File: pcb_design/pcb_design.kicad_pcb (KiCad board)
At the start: 2 copper layers, 37 parts, among them J1 USB_C_Receptacle_USB2.0_16P, J2 JST_PH_S2B-PH-K, J3 JST_PH_S2B-PH-K, J4 JST_PH_S2B-PH-K, Q1 MMBT3904, Q2 MMBT3904, SW1 SW_SPDT, U1 AP2112K-3.3, U2 ESP32-C3-WROOM-02, U3 MPU-6050, U4 QMC6308, U5 AP2112K-1.8, U6 TXS0102DCU, U7 MCP73831-2-OT

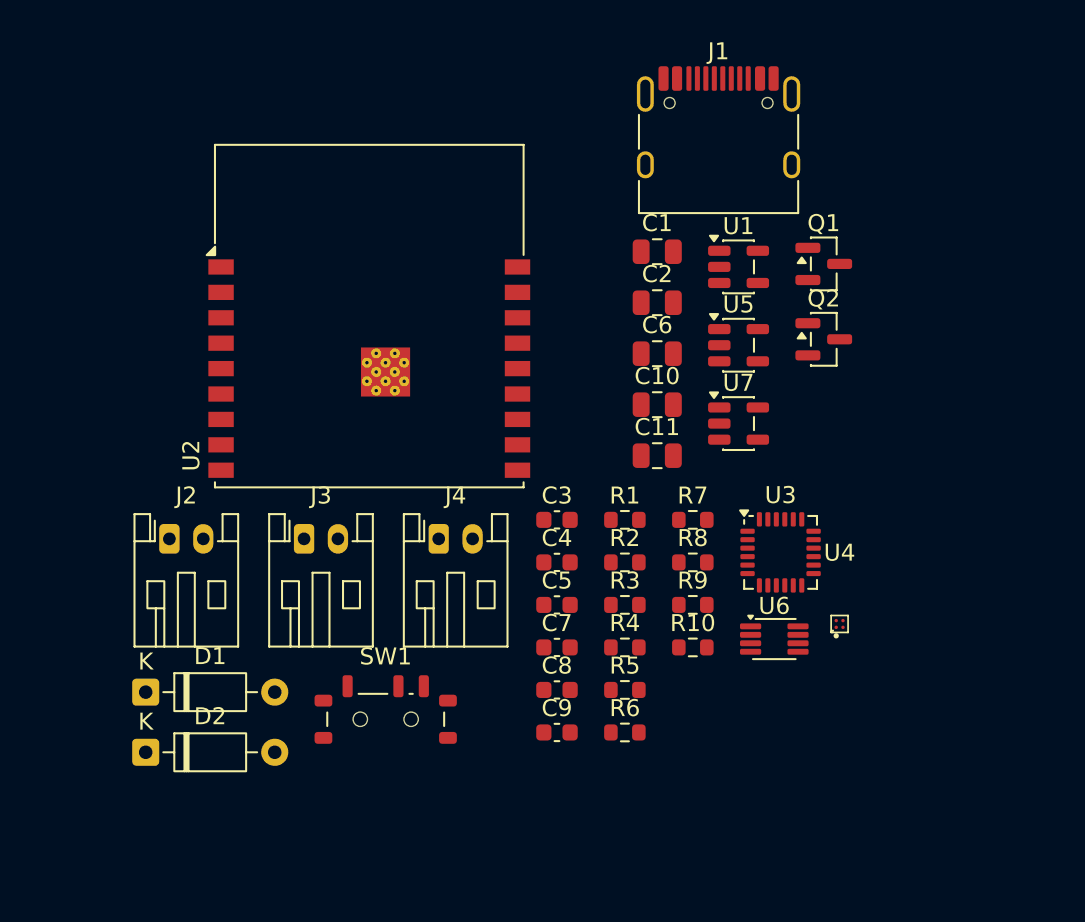
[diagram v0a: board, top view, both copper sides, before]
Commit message: feat: implement complete pcb design
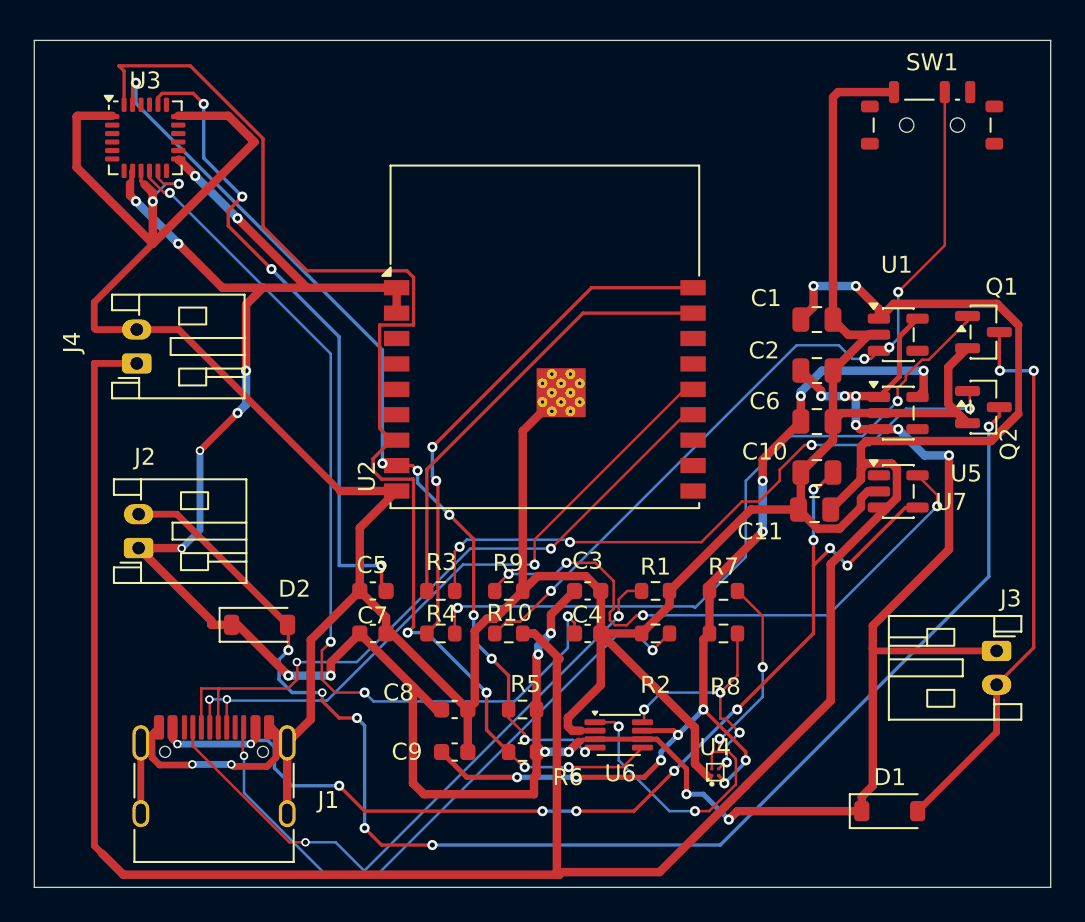
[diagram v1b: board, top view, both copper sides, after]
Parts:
- D1, D2: value 1N4148 -> 1N4148W; footprint Diode_THT:D_DO-35_SOD27_P7.62mm_Horizontal -> Diode_SMD:D_SOD-123
- moved J1 48.5 mm to (135.6, 118.6)
- moved SW1 47.7 mm to (178.0, 79.0)
- moved U3 44.8 mm to (131.6, 79.8)
- moved D1 44.5 mm to (175.5, 119.5)
- moved J3 41.4 mm to (181.8, 110.0), turned to -90 degrees
- moved J4 20.6 mm to (131.1, 93.1), turned to 90 degrees
- moved U4 11.4 mm to (165.2, 117.2)
- moved R10 10.9 mm to (153.0, 109.0)
- moved R3 10.9 mm to (149.0, 106.5)
- moved R4 10.9 mm to (149.0, 109.0)
- moved R9 10.9 mm to (153.0, 106.5)
- moved C5 10.9 mm to (145.0, 106.5)
- moved C7 10.9 mm to (145.0, 109.0)
- moved U6 10.8 mm to (159.5, 115.0)
- moved U2 10.4 mm to (155.1, 94.6)
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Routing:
- net GND: track 0.00 -> 230.1 mm, vias 0 -> 4
- net /+3.3V: track 0.00 -> 173.6 mm, vias 0 -> 22
- net /VBAT: track 0.00 -> 149.7 mm, vias 0 -> 2
- net Net-(D2-A): track 0.00 -> 81.6 mm, vias 0 -> 6
- net Net-(U2-IO8): track 0.00 -> 73.2 mm, vias 0 -> 4
- net /VBUS: track 0.00 -> 65.1 mm, vias 0 -> 11
- net /+1.8V: track 0.00 -> 57.3 mm, vias 0 -> 11
- net Net-(U2-IO9): track 0.00 -> 55.2 mm, vias 0 -> 8
- net Net-(U3-REGOUT): track 0.00 -> 54.5 mm, vias 0 -> 4
- net Net-(SW1-B): track 0.00 -> 47.4 mm, vias 0 -> 4
- net Net-(Q1-B): track 0.00 -> 42.3 mm, vias 0 -> 2
- net Net-(U2-IO18): track 0.00 -> 41.0 mm, vias 0 -> 2
- net Net-(U2-IO19): track 0.00 -> 40.4 mm, vias 0 -> 3
- net Net-(U3-CPOUT): track 0.00 -> 38.8 mm, vias 0 -> 4
- net Net-(J1-CC1): track 0.00 -> 38.1 mm, vias 0 -> 2
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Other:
- board outline added: 60 x 50 mm
